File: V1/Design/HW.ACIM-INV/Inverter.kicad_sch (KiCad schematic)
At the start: 59 parts, among them J3 MOTOR, M1 560V/1.75kA, M2 560V/1.75kA, M3 560V/1.75kA, Q4 20V/1A, Q5 20V/1A, Q6 20V/1A, U1 IPM 600V/15A, U15 I=±10A, U16 I=±10A

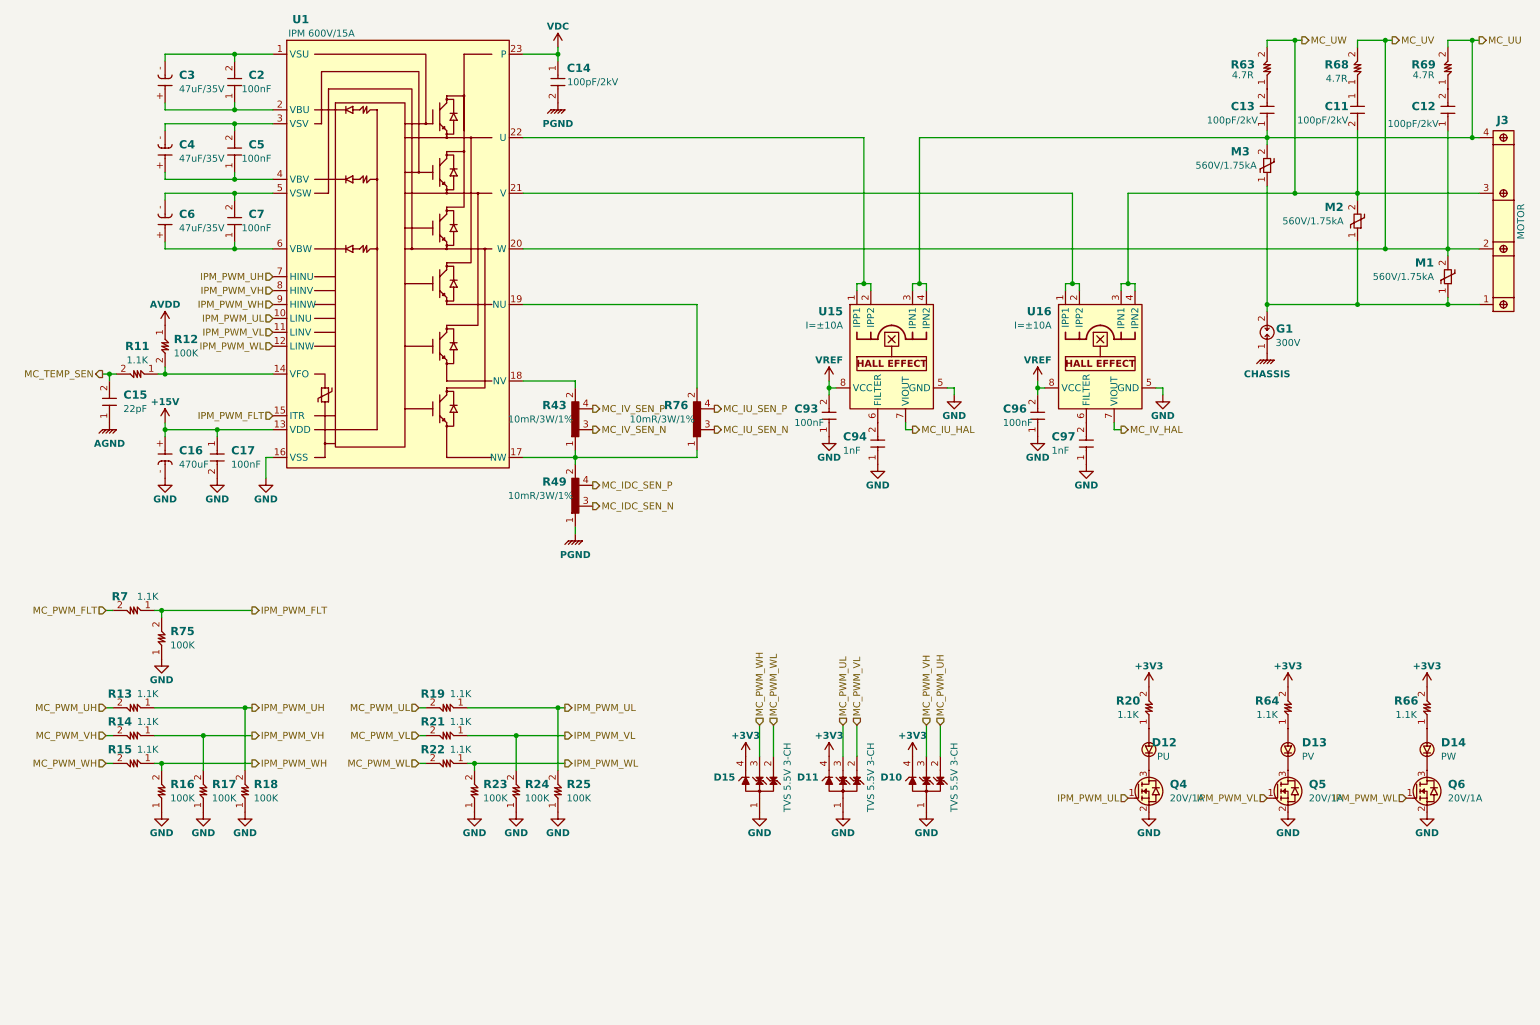
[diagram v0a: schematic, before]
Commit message: V1 schematic update 11
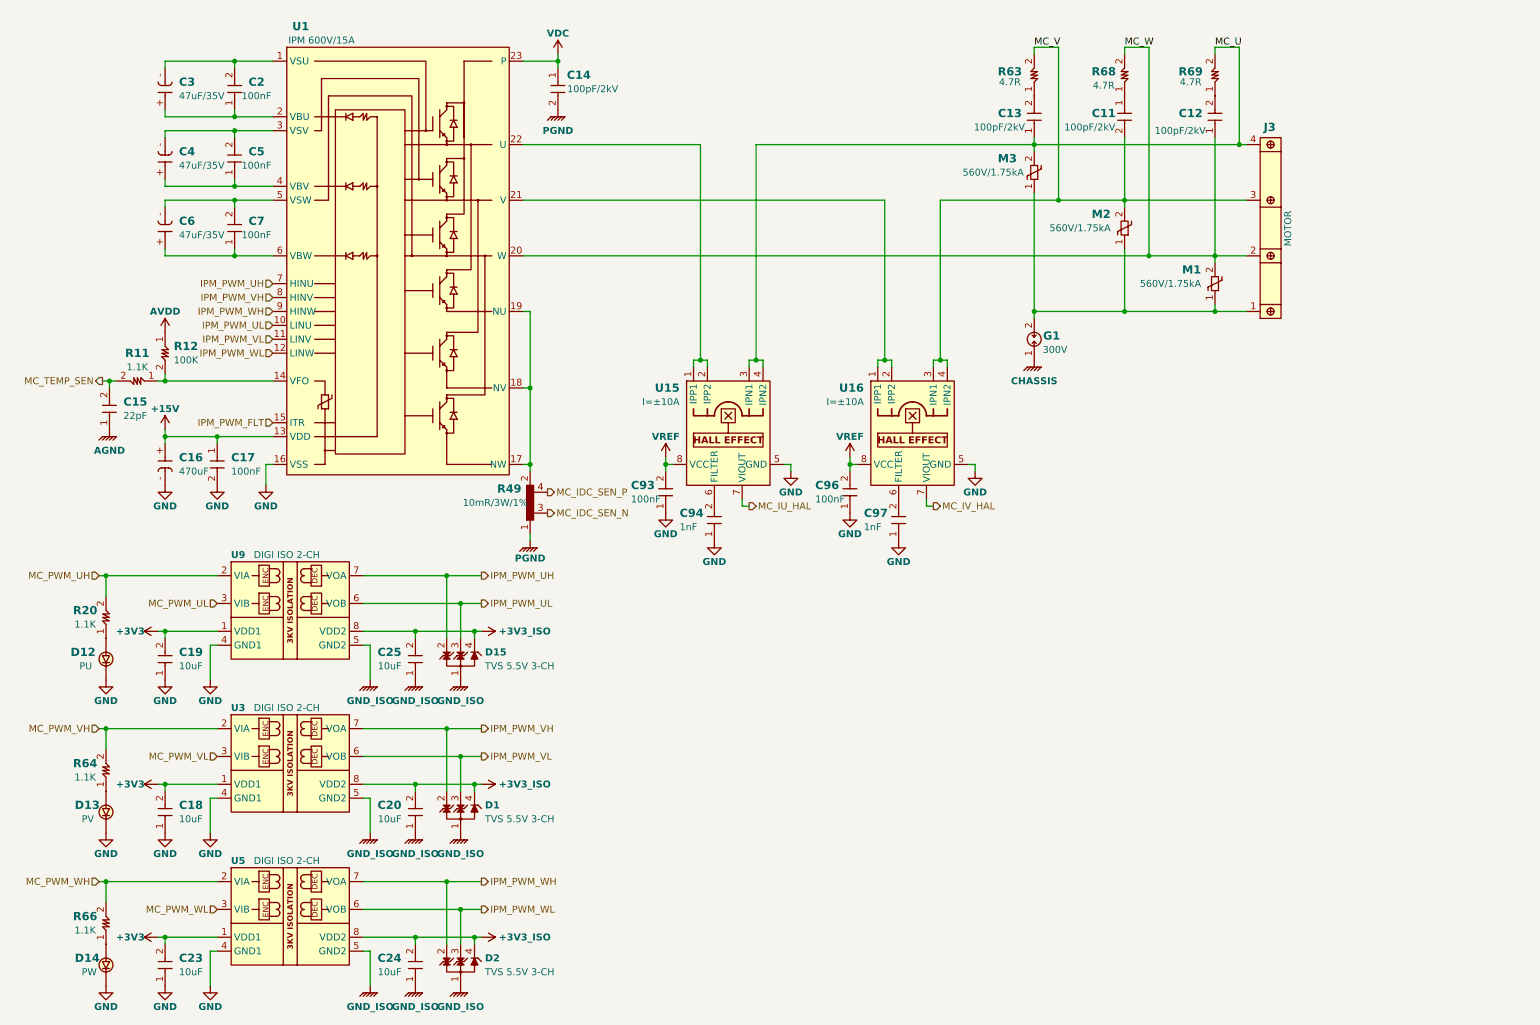
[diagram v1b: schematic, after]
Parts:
- removed D10, D11: TVS 5.5V 3-CH, SAMPI:SOT143B_NEXT, symbol SAM1:TVS_3CH
- removed Q4, Q5, Q6: 20V/1A, SAMPI:SOT23, symbol SAMPI:FET_N-CH
- removed R13, R14, R15, R19, R21, R22, R7: 1.1K, SAMPI:RES0603, symbol SAMPI:RES
- removed R16, R17, R18, R23, R24, R25, R75: 100K, SAMPI:RES0603, symbol SAMPI:RES
- removed R43, R76: 10mR/3W/1%, SAMPI:SHU2512, symbol SAMPI:SHUNT
- added C18, C19, C20, C23, C24, C25: 10uF, SAMPI:CAP0603, symbol SAMPI:CERCAP
- added D1, D2: TVS 5.5V 3-CH, SAMPI:SOT143B_NEXT, symbol SAM1:TVS_3CH
- added U3, U5, U9: DIGI ISO 2-CH, SAMPI:SOIC8_ALL, symbol SAMPI:ADUM1200
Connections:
- net +3V3: now also C18.2, C19.2, C23.2, U3.1 (VDD1), U5.1 (VDD1), U9.1 (VDD1); no longer D15.4 (CH3), R20.2, R64.2, R66.2
- net GND: now also D12.K, D13.K, D14.K, C18.1, C19.1, C23.1, U3.4 (GND1), U5.4 (GND1), U9.4 (GND1); no longer D15.1 (GND)
- net IPM_PWM_UH: now also D15.2 (CH1), U9.7 (VOA)
- net IPM_PWM_UL: now also D15.3 (CH2), U9.6 (VOB)
- net IPM_PWM_VH: now also D1.2 (CH1), U3.7 (VOA)
- net IPM_PWM_VL: now also D1.3 (CH2), U3.6 (VOB)
- net IPM_PWM_WH: now also D2.2 (CH1), U5.7 (VOA)
- net IPM_PWM_WL: now also D2.3 (CH2), U5.6 (VOB)
- net MC_PWM_UH: now also R20.2, U9.2 (VIA)
- net MC_PWM_UL: now also U9.3 (VIB)
- net MC_PWM_VH: now also R64.2, U3.2 (VIA)
- net MC_PWM_VL: now also U3.3 (VIB)
- net MC_PWM_WH: now also R66.2, U5.2 (VIA); no longer D15.3 (CH2)
- net MC_PWM_WL: now also U5.3 (VIB); no longer D15.2 (CH1)
- net at R49.2, U1.17 (NW): now also U1.18 (NV), U1.19 (NU)
- net MC_UU renamed MC_U
- net MC_UV renamed MC_W
- net MC_UW renamed MC_V
- new net +3V3_ISO: C20.2, C24.2, C25.2, D1.4 (CH3), D15.4 (CH3), D2.4 (CH3), U3.8 (VDD2), U5.8 (VDD2), U9.8 (VDD2)
- new net GND_ISO: C20.1, C24.1, C25.1, D1.1 (GND), D15.1 (GND), D2.1 (GND), U3.5 (GND2), U5.5 (GND2), U9.5 (GND2)
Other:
- moved on the sheet: C11, C12, C13, C14, C15, C16, C17, C2, C3, C4, C5, C6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
